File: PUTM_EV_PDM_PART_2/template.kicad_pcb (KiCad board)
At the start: 4 copper layers, 60 x 90 mm, 7 parts, among them J3 Conn_02x18_Counter_Clockwise, J4 WIRE OUT, J5 Conn_01x37

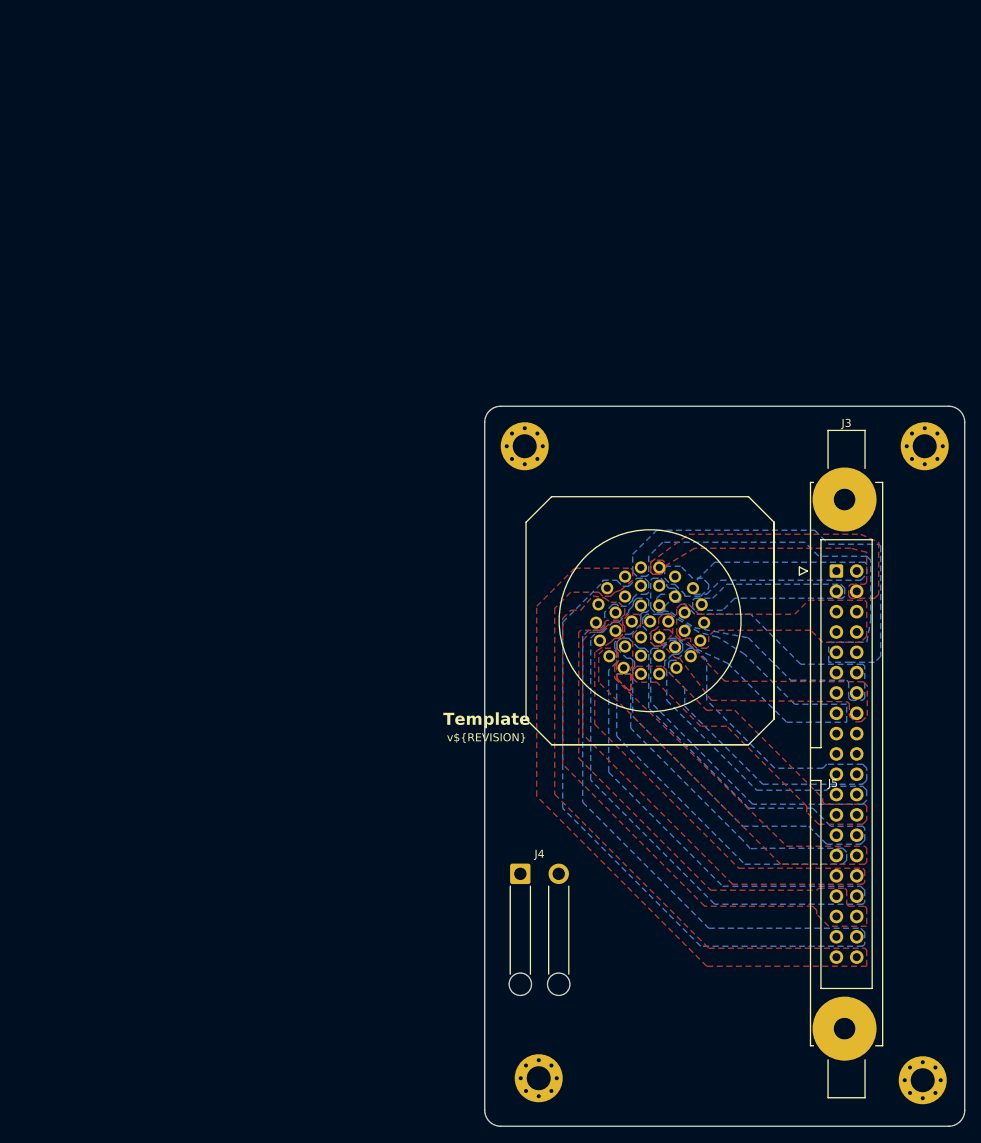
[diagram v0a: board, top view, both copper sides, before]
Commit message: Add files via upload
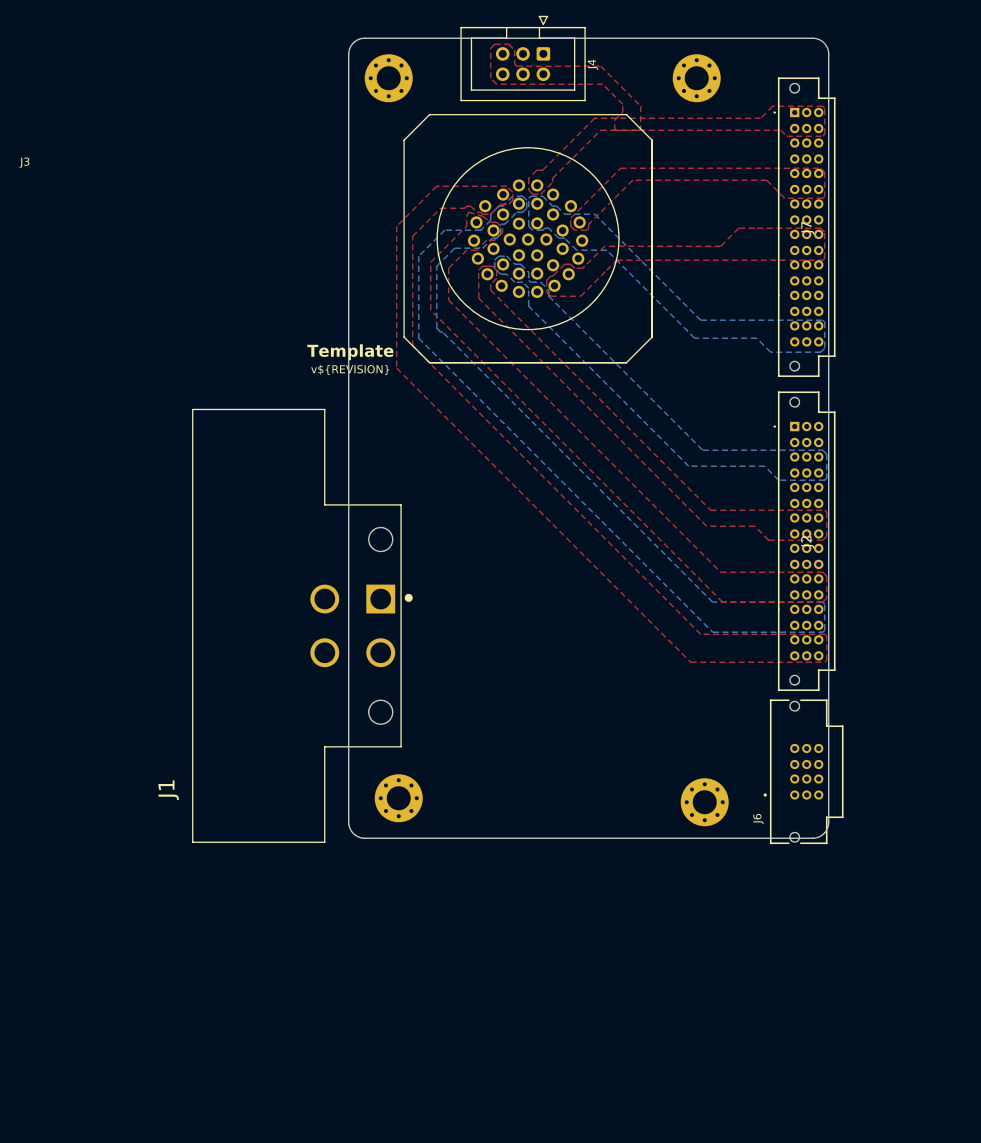
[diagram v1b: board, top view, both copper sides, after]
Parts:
- removed J5: Conn_01x37, 3RD_party:37 PIN DEUTSCH
- added J1: +24V IN, DPT13-4P:TE_DTP13-4P, F.Cu at (103.0, 103.5)
- added J2: UPS-08-07.0-01-L-V, UPT-08-07-01-L-V:UPS0807001LV, F.Cu at (154.8, 78.5)
- added J6: +24V OUT, UPT-02-01-01-L-V:SAMTEC_UPT-02-03.0-XX-X-V, F.Cu at (156.2, 121.7)
- added J7: UPS-08-07.0-01-L-V, UPT-08-07-01-L-V:UPS0807001LV, F.Cu at (154.8, 39.3)
- J3: footprint Connector_IDC:IDC-Header_2x20-1MP_P2.54mm_Latch6.5mm_Vertical -> 3RD_party:37 PIN DEUTSCH
- J4: value WIRE OUT -> Conn_01x06_Pin; footprint Connector_Wire:SolderWire-0.75sqmm_1x02_P4.8mm_D1.25mm_OD2.3mm_Relief -> Connector_IDC:IDC-Header_2x03_P2.54mm_Vertical
- moved J4 102.5 mm to (123.3, 32.0), turned to -90 degrees
- moved J3 56.7 mm to (121.4, 55.1)
- moved xd1 54.1 mm to (142.5, 35.0)
- moved xd2 49.0 mm to (104.0, 35.0)
- moved xd4 44.2 mm to (143.5, 125.5)
- moved xd3 39.1 mm to (105.2, 125.0)
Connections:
- J3 pad 15: /DASH 24VDC -> /BRAKE BALANCE 24VDC
- J3 pad 17: /PC 24VDC 4 -> /PC 24VDC 3
- J3 pad 19: /TSAL LOGIC 24VDC -> /BSPD 24VDC
- J3 pad 20: /TSAL LIGHT 24VDC -> /BSPD 24VDC
- J3 pad 21: /DIAGPORT 24VDC -> /AIR PRESSURE 24VDC
- J3 pad 22: /IR CAMS REAR 24VDC -> /AIR PRESSURE 24VDC
- J3 pad 24: /ODRIVE 3 24VDC -> /ODRIVE 2 24VDC
- J3 pad 26: /ODRIVE 5 24VDC -> /ODRIVE 4 24VDC
- J3 pad 27: /PC 24VDC 2 -> /PC 24VDC 1
- J3 pad 28: /FRONT BOX 24VDC -> /BRAKE BALANCE 24VDC
- J3 pad 3: /REARBOX 2 24VDC -> /REARBOX 1 24VDC
- J3 pad 30: /INVERTER 2 24VDC -> /INVERTER 1 24VDC
- J3 pad 33: /HV LOGIKA 2 24VDC -> /HV LOGIKA 1 24VDC
- J3 pad 6: /IR CAMS FRONT 24VDC -> /AIR PRESSURE 24VDC
- J3 pad 8: /REARBOX 4 24VDC -> /REARBOX 3 24VDC
- J3 pad 9: /SDC SOURCE -> /ASMS SOURCE
- J4 pad 1: /+24V -> /CAN_L
- J4 pad 2: /GND -> /CAN_H
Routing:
- added copper zone on In1.Cu, net (none)
- added copper zone on In2.Cu, net (none)
- added copper zone on F.Cu, net /AIR PRESSURE 24VDC
- added copper zone on In2.Cu, net /ASMS IN
- added copper zone on In2.Cu, net /ASMS SOURCE
- added copper zone on F.Cu, net /BRAKE BALANCE 24VDC
- added copper zone on In1.Cu, net /CAN_L
- added copper zone on B.Cu, net /ODRIVE 4 24VDC
- removed copper zone on B.Cu, net /ASMS IN
- removed copper zone on F.Cu, net /ASMS IN
- removed copper zone on F.Cu, net /ASMS SOURCE
- removed copper zone on B.Cu, net /CAN_H
- removed copper zone on B.Cu, net /CAN_L
- removed copper zone on F.Cu, net /DASH 24VDC
- removed copper zone on F.Cu, net /DIAGPORT 24VDC
- removed copper zone on F.Cu, net /HV LOGIKA 1 24VDC
- removed copper zone on B.Cu, net /ODRIVE 2 24VDC
- removed copper zone on B.Cu, net /ODRIVE 5 24VDC
- removed copper zone on F.Cu, net /PC 24VDC 1
- removed copper zone on B.Cu, net /REARBOX 1 24VDC
- removed copper zone on B.Cu, net /REARBOX 3 24VDC
- removed copper zone on B.Cu, net /REARBOX 5 24VDC
- removed copper zone on B.Cu, net /TSAL LIGHT 24VDC
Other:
- board size 60 x 90 mm -> 60 x 100 mm
